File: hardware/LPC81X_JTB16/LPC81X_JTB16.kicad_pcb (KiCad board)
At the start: 2 copper layers, 2 parts

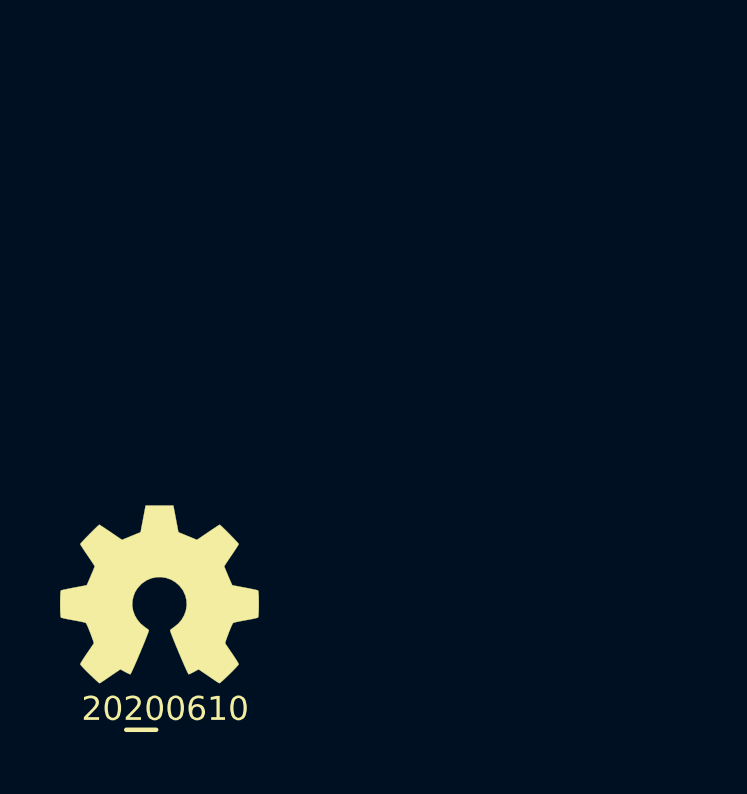
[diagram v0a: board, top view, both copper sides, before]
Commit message: WIP schematic definition and raw component placement
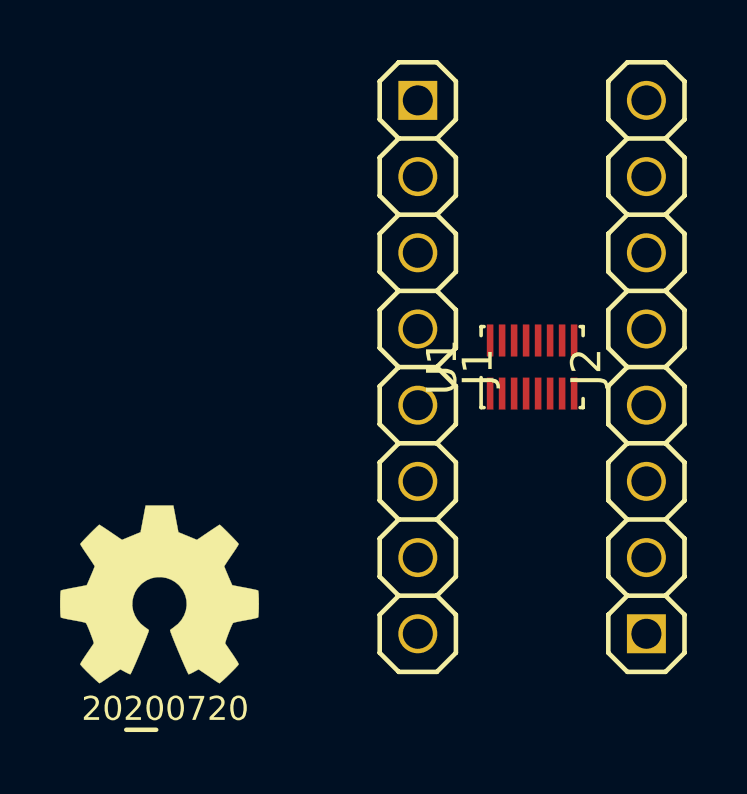
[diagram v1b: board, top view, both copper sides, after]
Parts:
- added J1: Conn_01x08, SquantorConnectors:Header-0254-1X08-H010, F.Cu at (147.3, 80.0)
- added J2: Conn_01x08, SquantorConnectors:Header-0254-1X08-H010, F.Cu at (154.9, 80.0)
- added U1: LPC812M101JTB16, Package_SON:NXP_XSON-16, F.Cu at (151.1, 80.0)
- N1: value 20200610 -> 20200720
